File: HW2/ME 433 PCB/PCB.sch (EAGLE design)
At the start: 22 parts, among them J1 USB-MB-H

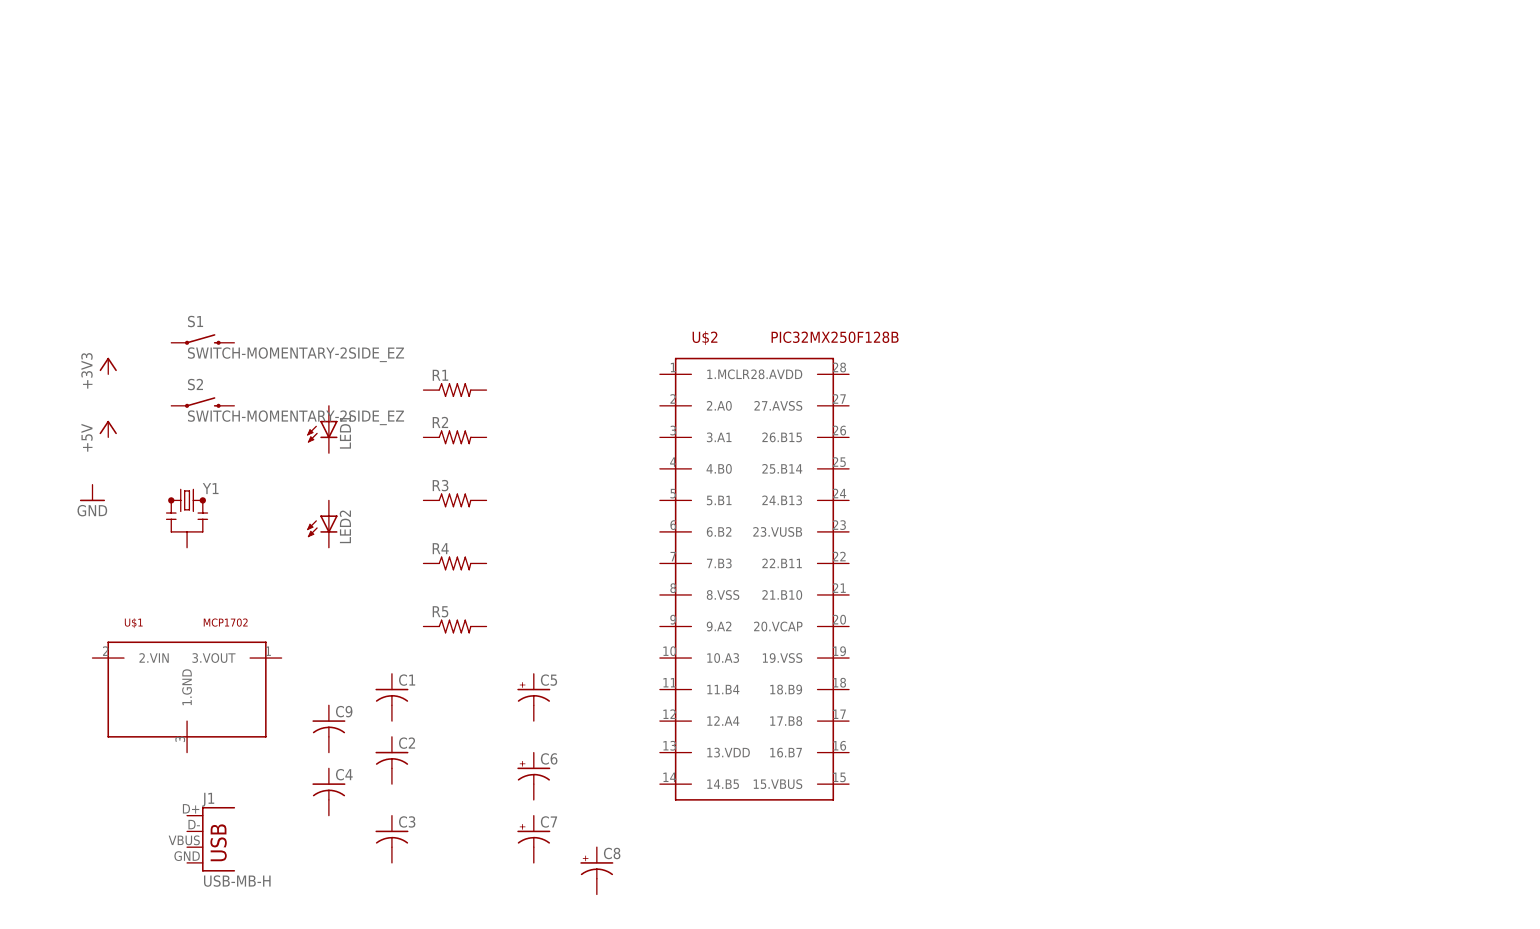
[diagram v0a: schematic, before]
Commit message: HW 2 Update
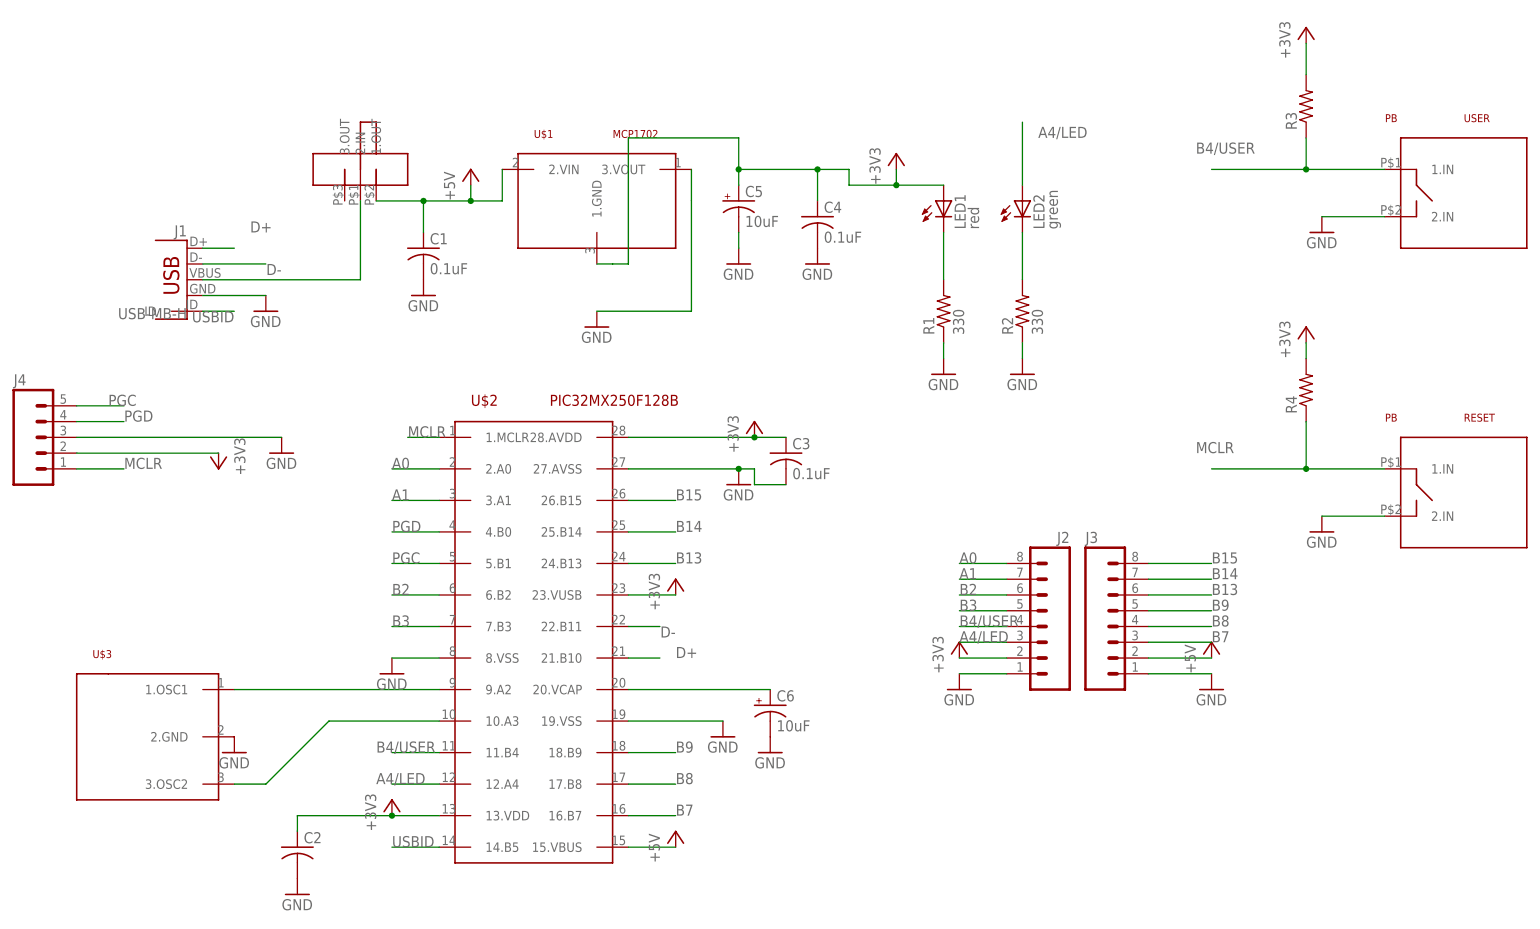
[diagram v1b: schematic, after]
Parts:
- removed C7, C8: (no value), ME 433 PCB lib:CPOL-USTAP5-60
- removed C9: (no value), ME 433 PCB lib:C-US025-025X050
- removed R5: (no value), ME 433 PCB lib:R-US_0207/10
- removed S1, S2: SWITCH-MOMENTARY-2SIDE_EZ, ME 433 PCB lib:SWITCH-MOMENTARY-2SIDE_EZ
- removed Y1: (no value), ME 433 PCB lib:RESONATORPTH
- added J2, J3: (no value), ME 433 PCB lib:M08
- added J4: (no value), ME 433 PCB lib:M05PTH
- added RESET, USER: PB, ME 433 PCB lib:PB
- added U$3: (no value), ME 433 PCB lib:CRES
- added U$5: SLIDE, ME 433 PCB lib:SLIDE
- C1, C3, C4: value (none) -> 0.1uF
- C5, C6: value (none) -> 10uF; device ME 433 PCB lib:CPOL-USTAP5-60 -> ME 433 PCB lib:CPOL-USB45181A
- LED1: value (none) -> red
- LED2: value (none) -> green
- R1, R2: value (none) -> 330
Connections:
- new net +3V3: C2.1, C3.1, C4.1, C5.+, J2.2, J4.2, LED1.A, R3.2, R4.2, U$1.1.GND, U$2.13.VDD, U$2.23.VUSB, U$2.28.AVDD
- new net +5V: C1.1, J3.2, U$1.2.VIN, U$2.15.VBUS, U$5.1.OUT
- new net A0: J2.8, U$2.2.A0
- new net A1: J2.7, U$2.3.A1
- new net A4/LED: J2.3, LED2.A, U$2.12.A4
- new net B13: J3.6, U$2.24.B13
- new net B14: J3.7, U$2.25.B14
- new net B15: J3.8, U$2.26.B15
- new net B2: J2.6, U$2.6.B2
- new net B3: J2.5, U$2.7.B3
- new net B4/USER: J2.4, R3.1, U$2.11.B4, USER.1.IN
- new net B7: J3.3, U$2.16.B7
- new net B8: J3.4, U$2.17.B8
- new net B9: J3.5, U$2.18.B9
- new net D+: J1.D+, U$2.21.B10
- new net D-: J1.D-, U$2.22.B11
- new net GND: C1.2, C2.2, C3.2, C4.2, C5.-, C6.-, J1.GND, J2.1, J3.1, J4.3, R1.1, R2.1, RESET.2.IN, U$1.3.VOUT, U$2.19.VSS, U$2.27.AVSS, U$2.8.VSS, U$3.2.GND, USER.2.IN
- new net MCLR: J4.1, R4.1, RESET.1.IN, U$2.1.MCLR
- new net N$1: J1.VBUS, U$5.2.IN
- new net N$29: C6.+, U$2.20.VCAP
- new net N$36: U$2.10.A3, U$3.3.OSC2
- new net N$37: U$2.9.A2, U$3.1.OSC1
- new net N$5: LED2.C, R2.2
- new net N$8: LED1.C, R1.2
- new net PGC: J4.5, U$2.5.B1
- new net PGD: J4.4, U$2.4.B0
- new net USBID: J1.ID, U$2.14.B5
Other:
- moved on the sheet: C1, C2, C3, C4, C5, C6, LED1, LED2, R1, R2, R3, R4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
